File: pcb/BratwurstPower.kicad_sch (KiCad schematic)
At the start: 39 parts, among them J1 BarrelJack, J10 GPIO, J11 OTG, J2 RaspiPower, J4 USB1out, J5 I2C, J6 I2C, J8 USB2out, J9 EXT, Q1 AO3401A, Q2 AO3401A, U1 PCA9557PW

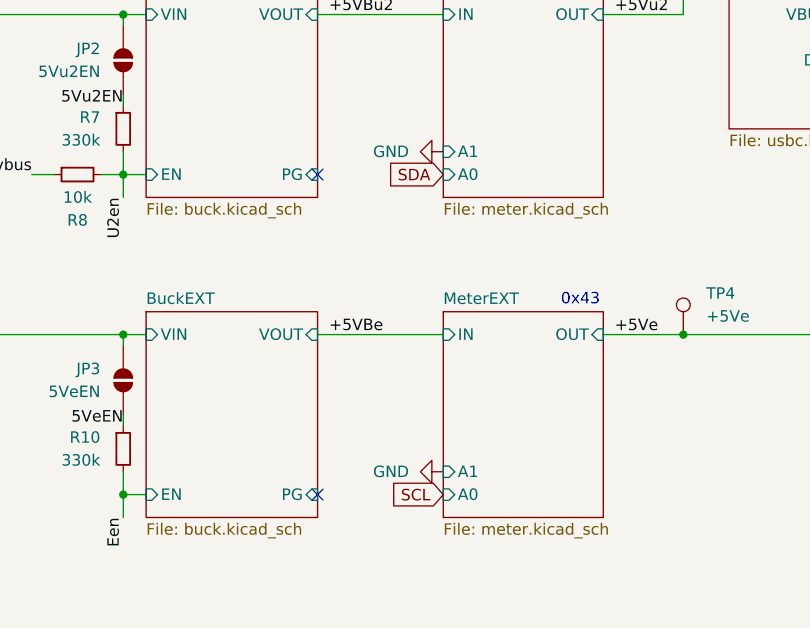
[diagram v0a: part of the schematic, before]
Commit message: chore: cleanup
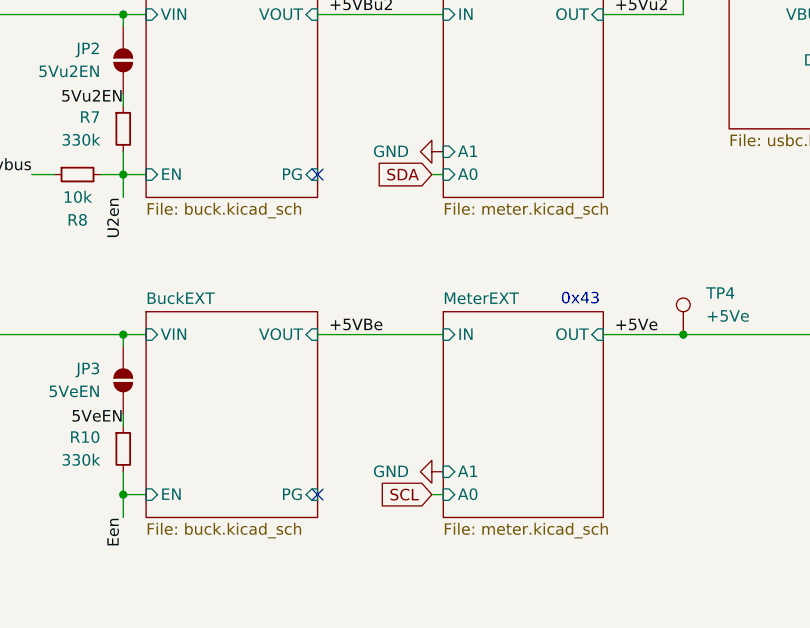
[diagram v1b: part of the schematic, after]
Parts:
- D6: footprint LED_SMD:LED_0805_2012Metric -> LED_SMD:LED_0603_1608Metric_Pad1.05x0.95mm_HandSolder
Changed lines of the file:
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@@
 	(wire
 		(pts
+			(xy 177.8 124.46) (xy 179.07 124.46)
+		)
+		(stroke
+			(width 0)
+			(type default)
+		)
+	)
+	(wire
+		(pts
 			(xy 33.02 85.09) (xy 33.02 72.39)
 		)
@@
 	(wire
 		(pts
+			(xy 177.8 160.02) (xy 179.07 160.02)
+		)
+		(stroke
+			(width 0)
+			(type default)
+		)
+	)
+	(wire
+		(pts
 			(xy 53.34 161.29) (xy 50.8 161.29)
 		)
@@
 	(global_label "SCL"
 		(shape input)
-		(at 179.07 160.02 180)
+		(at 177.8 160.02 180)
 		(fields_autoplaced yes)
 		(effects
@@
 		)
 		(property "Intersheetrefs" "${INTERSHEET_REFS}"
-			(at 172.5772 160.02 0)
+			(at 171.3072 160.02 0)
 			(effects
 				(font
@@
 	(global_label "SDA"
 		(shape input)
-		(at 179.07 124.46 180)
+		(at 177.8 124.46 180)
 		(fields_autoplaced yes)
 		(effects
@@
 		)
 		(property "Intersheetrefs" "${INTERSHEET_REFS}"
-			(at 172.5167 124.46 0)
+			(at 171.2467 124.46 0)
 			(effects
 				(font
@@
 			)
 		)
-		(property "Footprint" "LED_SMD:LED_0805_2012Metric"
+		(property "Footprint" "LED_SMD:LED_0603_1608Metric_Pad1.05x0.95mm_HandSolder"
 			(at 81.28 130.81 90)
 			(effects
